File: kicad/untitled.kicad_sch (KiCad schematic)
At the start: 26 parts, among them J3 Conn_Coaxial, J4 Conn_Coaxial, J5 SIM_Card, J6 Conn_02x20_Odd_Even, J7 Screw_Terminal_01x04, J8 Micro_SD_Card, Q3 NPN, SW1 SW_Push, SW2 SW_Push, U10 MAX3485, U5 ESP32-S3-WROOM-1, U7 SIM7080G, U8 TXS0102DCT

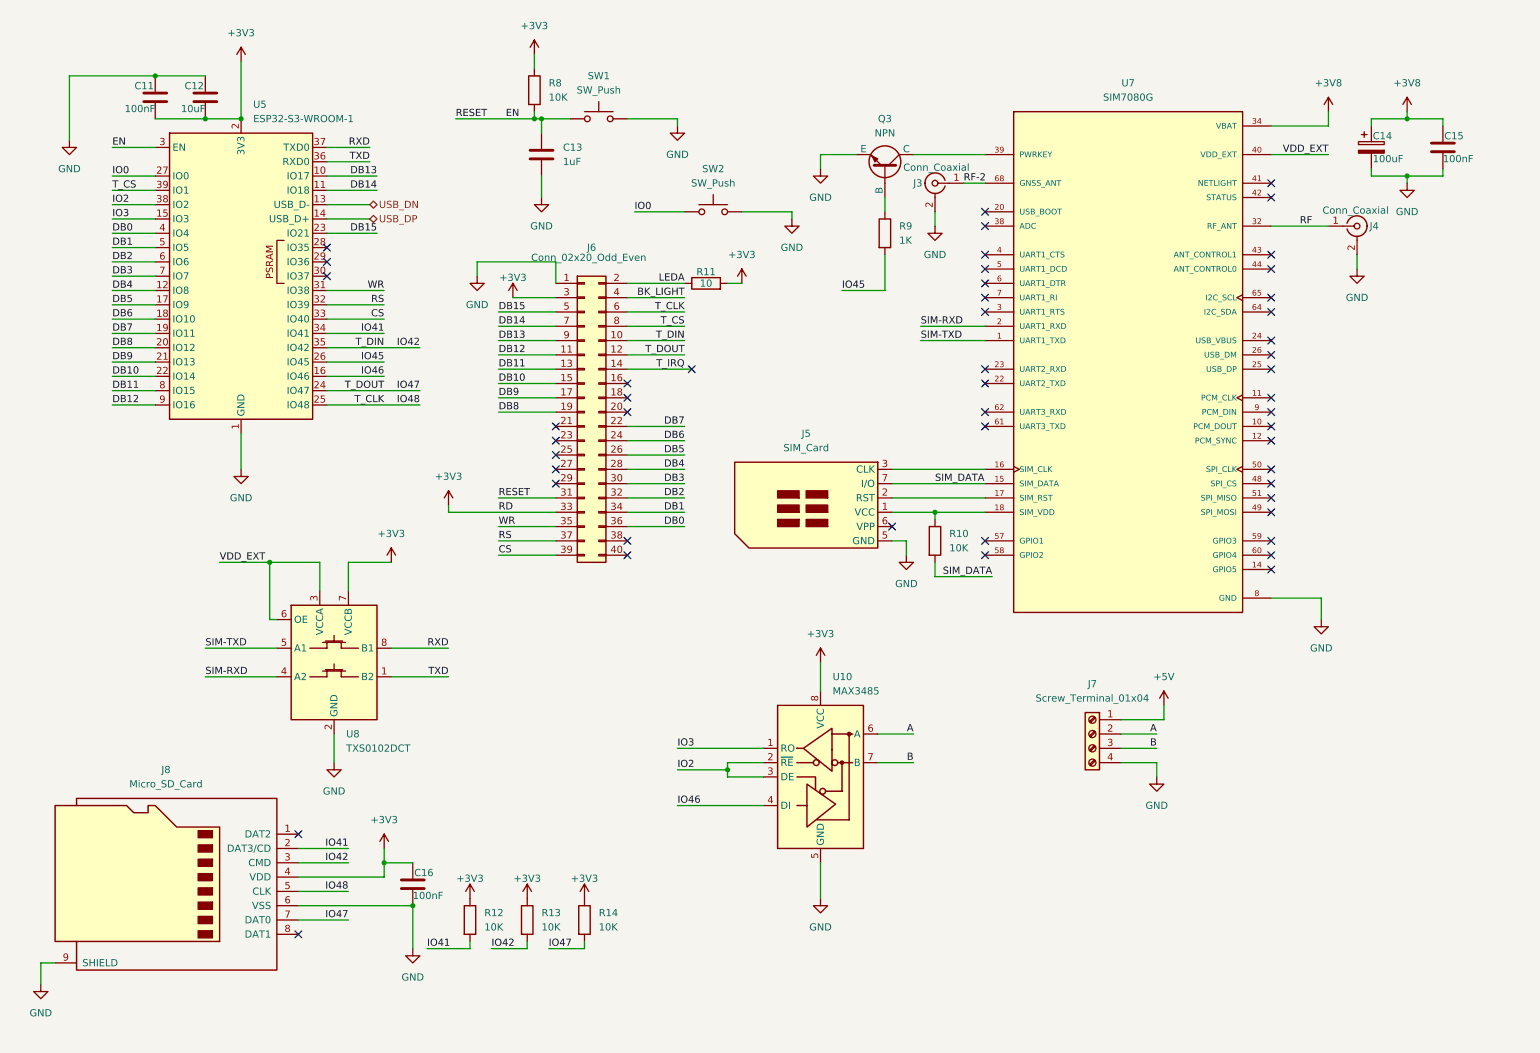
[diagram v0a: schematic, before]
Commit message: Completed the PCB
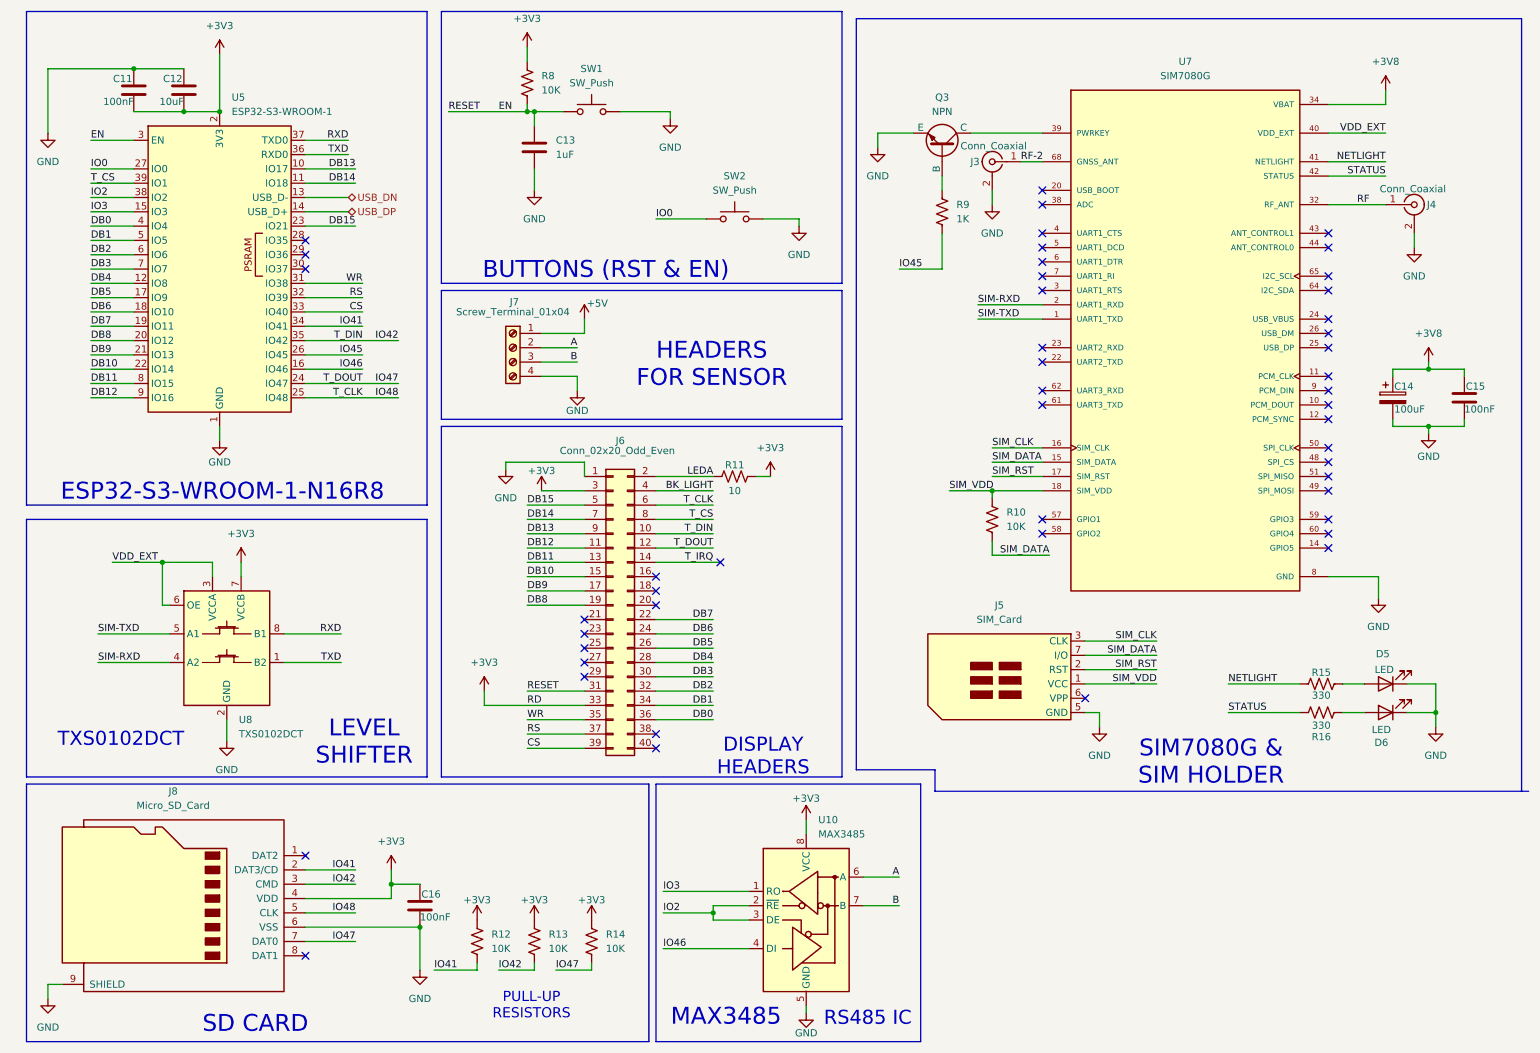
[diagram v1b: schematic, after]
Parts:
- added D5, D6: LED, LED_SMD:LED_0805_2012Metric_Pad1.15x1.40mm_HandSolder, symbol Device:LED
- added R15, R16: 330, Resistor_SMD:R_0805_2012Metric_Pad1.20x1.40mm_HandSolder, symbol Device:R
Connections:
- net GND: now also D5.1 (K), D6.1 (K)
- net SIM_CLK: now reaches J5.3 (CLK), U7.16 (SIM_CLK)
- net SIM_RST: now reaches J5.2 (RST), U7.17 (SIM_RST)
- net SIM_VDD: now reaches J5.1 (VCC), R10.1, U7.18 (SIM_VDD)
- net NETLIGHT: now reaches U7.41 (NETLIGHT)
- net NETLIGHT: now also R15.1
- net STATUS: now reaches U7.42 (STATUS)
- net STATUS: now also R16.1
- new net: D5.2 (A), R15.2
- new net: D6.2 (A), R16.2
- no-connect marks 50 -> 48
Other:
- note added: "BUTTONS (RST & EN)"
- note added: "DISPLAY HEADERS"
- note added: "ESP32-S3-WROOM-1-N16R8"
- note added: "HEADERS FOR SENSOR"
- note added: "LEVEL SHIFTER"
- note added: "MAX3485"
- note added: "PULL-UP RESISTORS"
- note added: "RS485 IC"
- note added: "SD CARD"
- note added: "SIM7080G & SIM HOLDER"
- note added: "TXS0102DCT"
- moved on the sheet: C11, C12, C13, C14, C15, C16, J3, J4, J6, J7, J8, Q3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
